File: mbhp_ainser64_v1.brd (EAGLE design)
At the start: 68.2 x 69.8 mm, 24 parts, among them IC1 MCP3208-CI/P, IC10 4051N, IC11 4051N, IC2 74HC595N, IC9 4051N, J11 1, J12 1, J13 1, J2 1

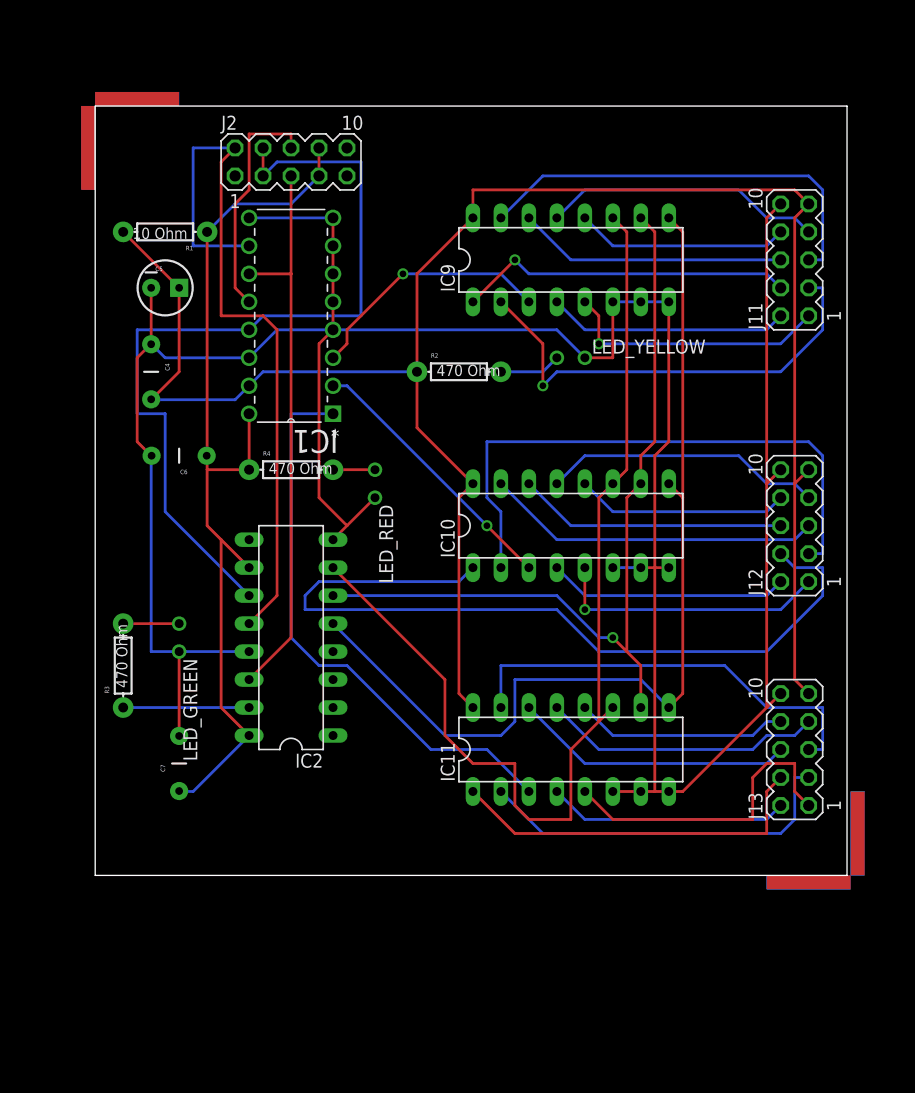
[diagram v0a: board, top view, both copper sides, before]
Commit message: design ready
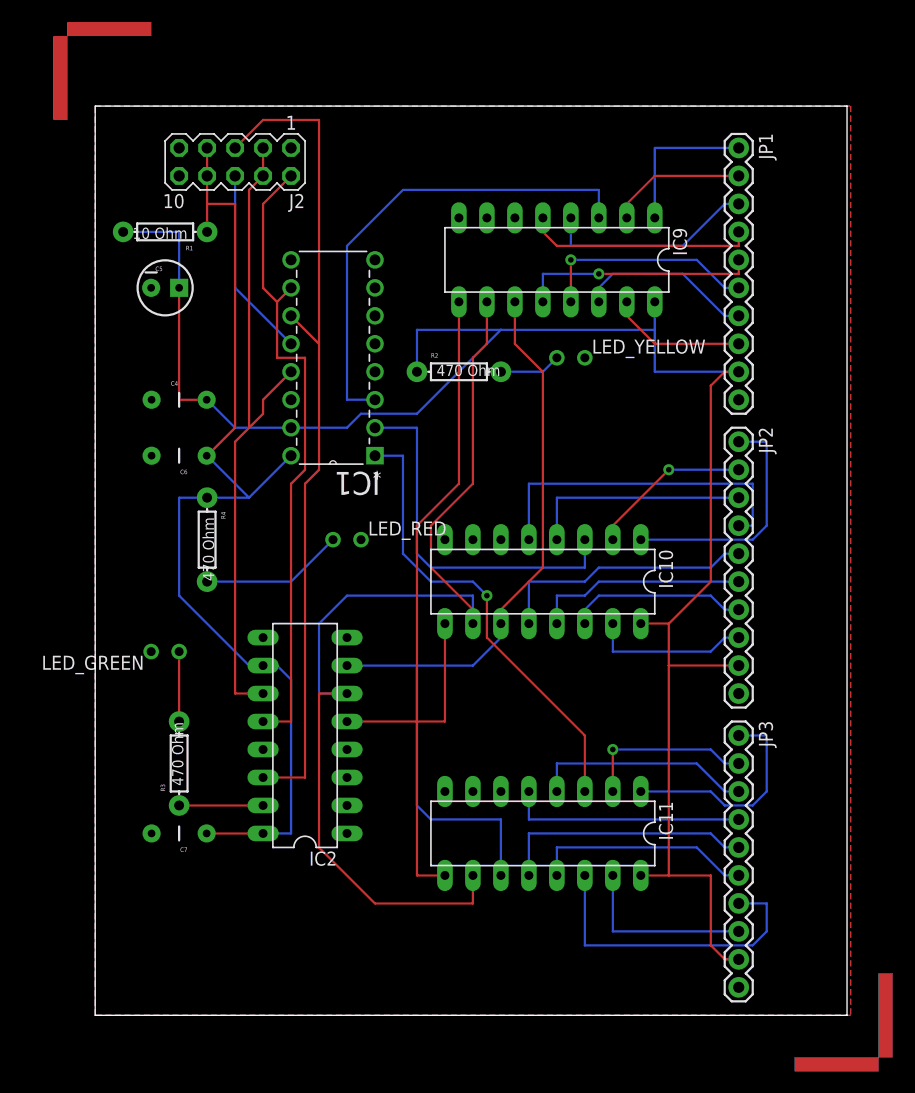
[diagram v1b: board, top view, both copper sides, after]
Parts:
- removed J11, J12, J13: 1, con-lstb:MA05-2
- added JP1, JP2, JP3: M10", SparkFun-Connectors:1X10
- moved U$2 16.7 mm to (77.5, -6.35)
- moved U$4 16.7 mm to (77.5, -6.35)
- moved R3 10.2 mm to (14.0, 20.3)
- moved R4 9.92 mm to (16.5, 40.6), turned to 270 degrees
- moved IC2 8.98 mm to (25.4, 22.9)
- moved IC11 8.03 mm to (47.0, 14.0), turned to 180 degrees
- moved U$1 6.84 mm to (3.81, 86.4)
- moved U$3 6.84 mm to (3.81, 86.4)
- moved C7 6.35 mm to (14.0, 14.0), turned to 180 degrees
- moved IC10 5.68 mm to (47.0, 36.8), turned to 180 degrees
- moved LED_RED 5.68 mm to (29.2, 40.6), turned to 0 degrees
- moved IC1 5.39 mm to (24.1, 66.0)
- moved J2 5.08 mm to (19.1, 74.9), turned to 180 degrees
- moved C4 3.59 mm to (14.0, 53.3), turned to 0 degrees
- moved LED_GREEN 1.80 mm to (12.7, 30.5), turned to 180 degrees
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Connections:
- net GND: now also JP1.10, JP2.10, JP3.10; no longer J11.10, J12.10, J13.10
- net N$10: now also IC10.14, JP2.7; no longer IC11.5, J13.1
- net N$11: now also IC10.15, JP2.8; no longer IC11.2, J13.3
- net N$12: now also IC10.12, JP2.5; no longer IC11.1, J13.4
- net N$13: now also IC10.5, JP2.4; no longer IC11.12, J13.8
- net N$14: now also IC10.4, JP2.3; no longer IC11.15, J13.5
- net N$15: now also IC10.2, JP2.2; no longer IC11.14, J13.6
- net N$16: now also IC10.1, JP2.1; no longer IC11.13, J13.7
- net N$17: now also IC11.15, JP3.8; no longer IC10.4, J12.2
- net N$18: now also IC11.14, JP3.7; no longer IC10.5, J12.1
- net N$19: now also IC11.13, JP3.6; no longer IC10.2, J12.3
- net N$20: now also IC11.12, JP3.5; no longer IC10.1, J12.4
- net N$21: now also IC11.5, JP3.4; no longer IC10.12, J12.8
- net N$22: now also IC11.4, JP3.3; no longer IC10.15, J12.5
- net N$23: now also IC11.2, JP3.2; no longer IC10.14, J12.6
- net N$24: now also IC11.1, JP3.1; no longer IC10.13, J12.7
- net N$25: now also IC9.15, JP1.8; no longer IC9.5, J11.1
- net N$26: now also IC9.14, JP1.7; no longer IC9.1, J11.4
- net N$27: now also IC9.13, JP1.6; no longer IC9.12, J11.8
- net N$28: now also IC9.12, JP1.5; no longer IC9.4, J11.2
- net N$29: now also IC9.5, JP1.4; no longer IC9.2, J11.3
- net N$30: now also IC9.4, JP1.3; no longer IC9.15, J11.5
- net N$31: now also IC9.2, JP1.2; no longer IC9.14, J11.6
- net N$32: now also IC9.1, JP1.1; no longer IC9.13, J11.7
- net N$6: now also JP1.9, JP2.9, JP3.9; no longer J11.9, J12.9, J13.9
- net N$9: now also IC10.13, JP2.6; no longer IC11.4, J13.2
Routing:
- net GND: track 265.0 -> 0.00 mm
- net N$20: track 75.1 -> 23.4 mm
- net N$19: track 53.1 -> 20.1 mm
- net N$3: track 51.1 -> 76.3 mm
- net CH2: track 22.7 -> 44.0 mm, vias 1 -> 0
- net MUXC: track 95.3 -> 74.1 mm
- net N$29: track 41.8 -> 20.8 mm, vias 1 -> 0
- net N$30: track 38.9 -> 19.4 mm
- net N$11: track 33.9 -> 14.5 mm
- net N$14: track 39.7 -> 20.3 mm
- net MUXB: track 75.3 -> 94.5 mm, vias 1 -> 0
- net N$2: track 76.6 -> 59.8 mm
- net N$26: track 30.6 -> 16.1 mm, vias 1 -> 0
- net MUXA: track 87.4 -> 74.0 mm
- net N$10: track 28.8 -> 16.3 mm
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- added copper zone on layer 1, net GND
- added copper zone on layer 16, net GND
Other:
- board size 68.2 x 69.8 mm -> 68.2 x 82.5 mm
